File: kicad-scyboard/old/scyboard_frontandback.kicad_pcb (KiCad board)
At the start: 2 copper layers, 144 x 96.5 mm, 92 parts

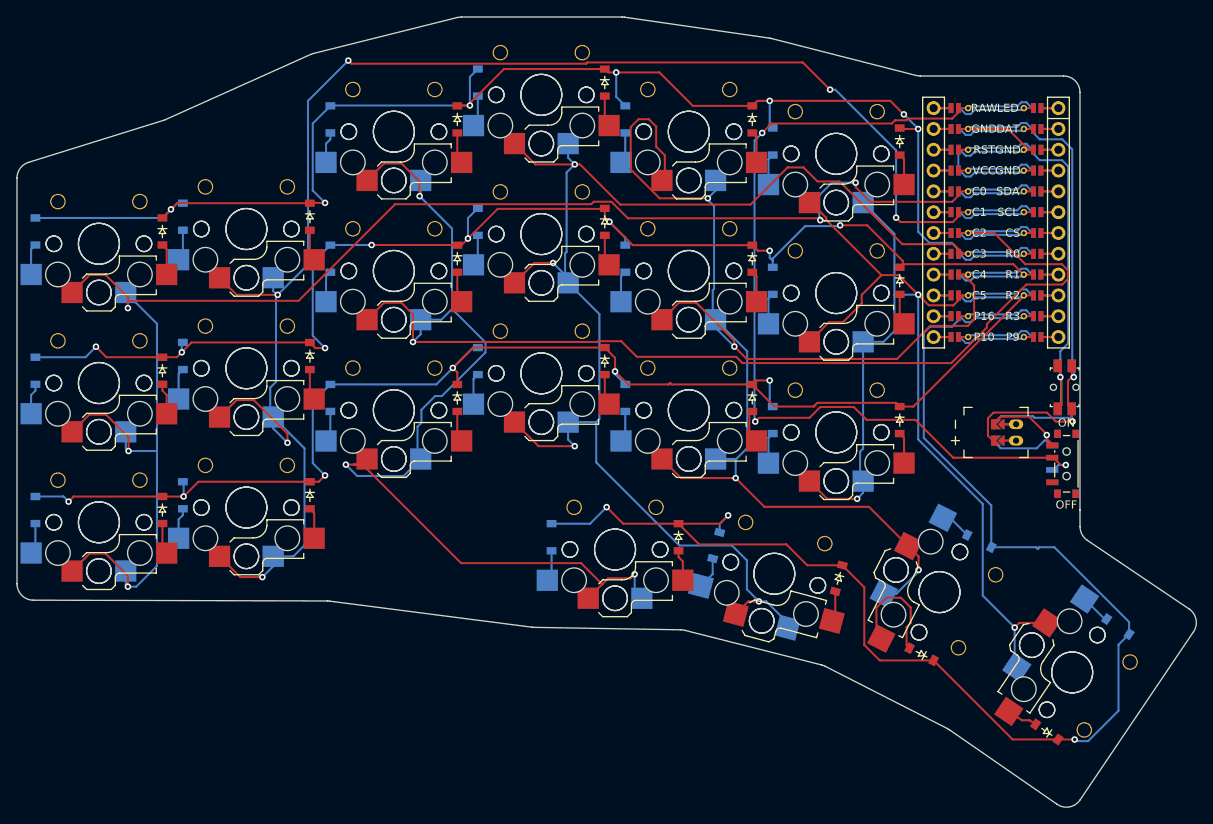
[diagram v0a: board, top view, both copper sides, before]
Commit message: Compile
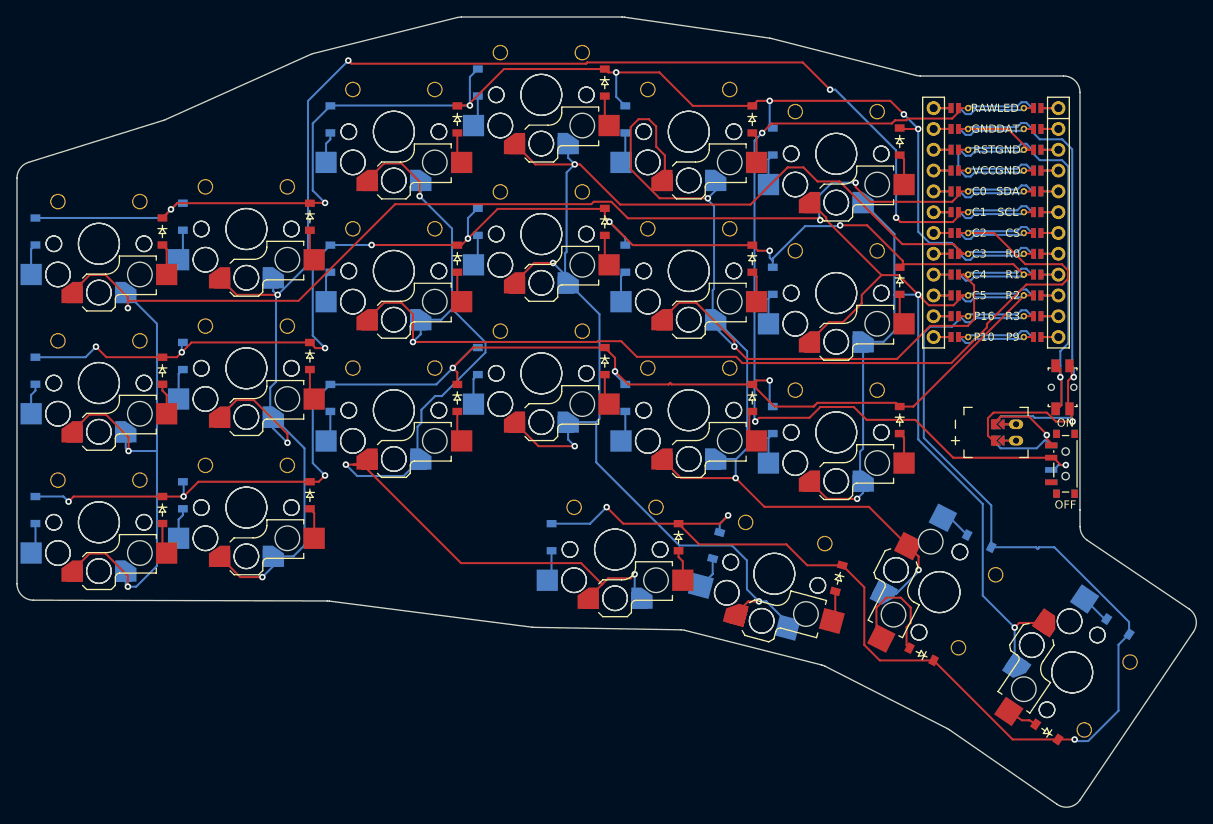
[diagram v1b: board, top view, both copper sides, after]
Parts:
- S1, S10, S11, S12, S13, S14, S15, S16, S17, S18, S19, S2, S21, S22, S3, S4, S5, S6, S7, S8, S9: footprint ceoloide:switch_choc_v1_v2 -> custom:custom_switch_choc_v1_v2_trimmed_b
- S23, S24, S25, S26, S27, S28, S29, S30, S31, S32, S33, S34, S35, S36, S37, S38, S39, S40, S41, S42, S44: footprint ceoloide:switch_choc_v1_v2 -> custom:custom_switch_choc_v1_v2_trimmed
- moved RST1 0.26 mm to (167.6, 83.5)
- moved PWR1 0.12 mm to (168.0, 92.9)
